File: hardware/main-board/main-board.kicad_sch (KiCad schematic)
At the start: 47 parts, among them J1 USB_C_Receptacle_USB2.0, J2 DNI, J3 Display Connector, U2 STM32L072KZT6, U4 USBLC6-2SC6, U5 TC1301A-APA

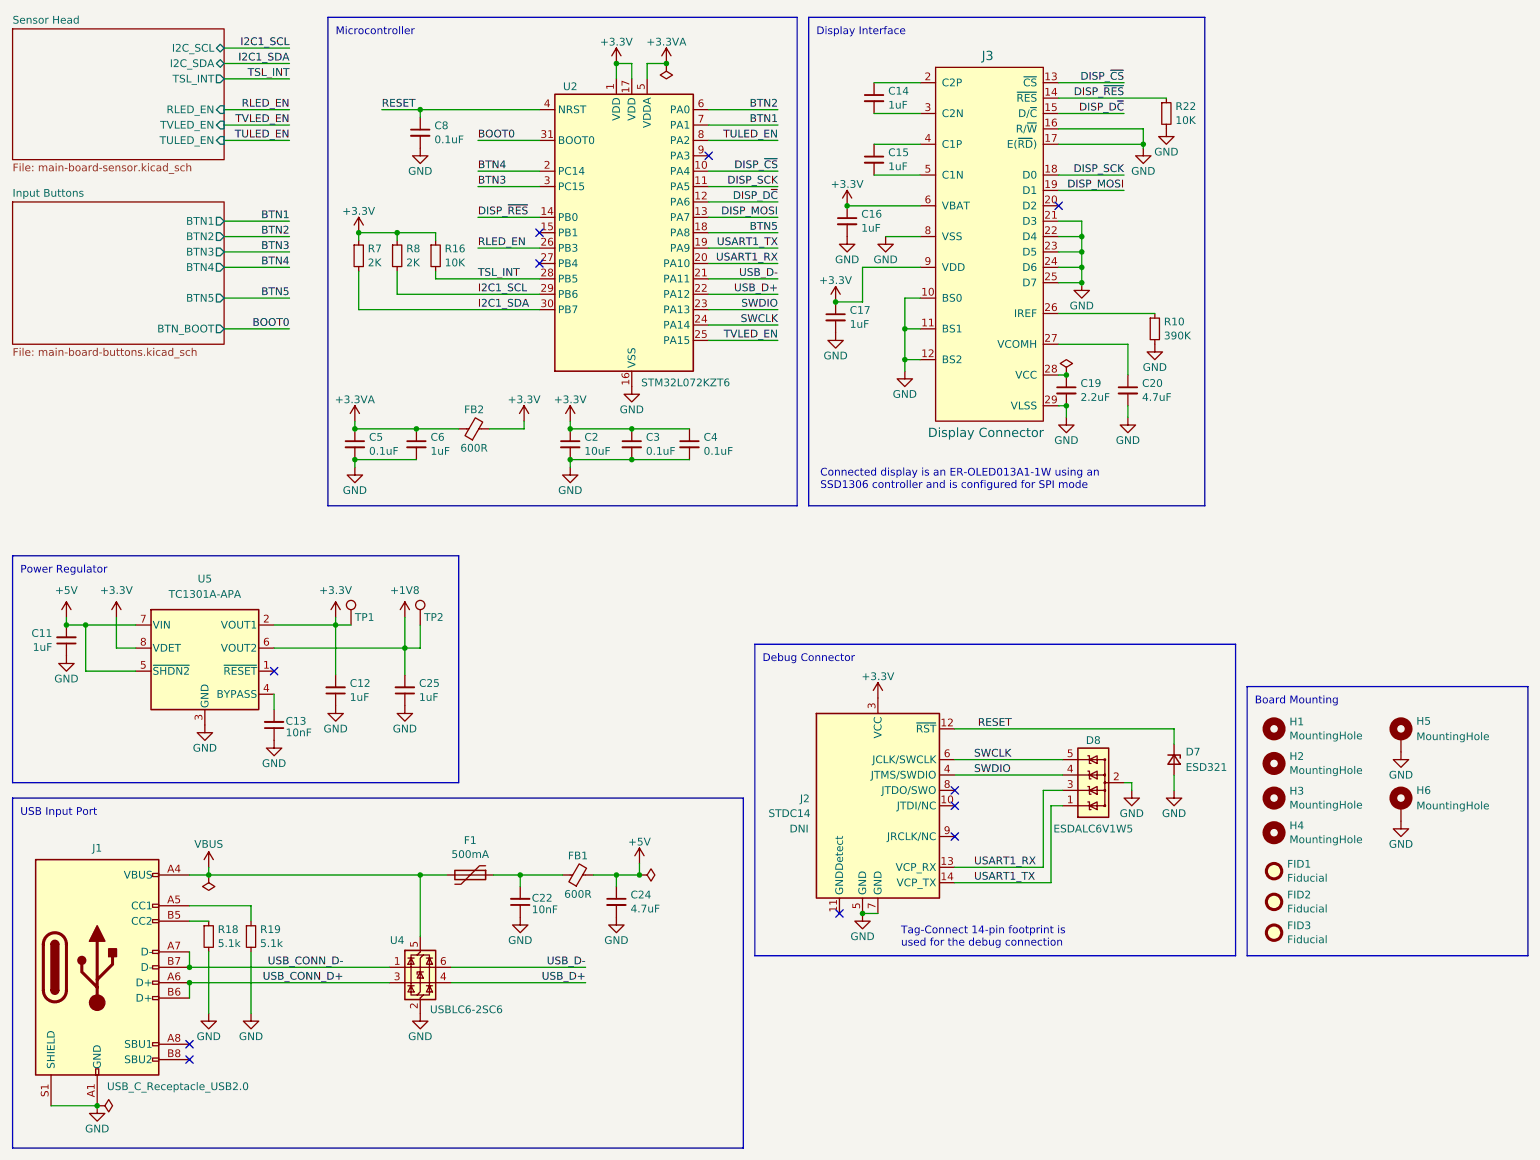
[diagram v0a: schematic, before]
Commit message: Final tweaks for Rev C manufacture
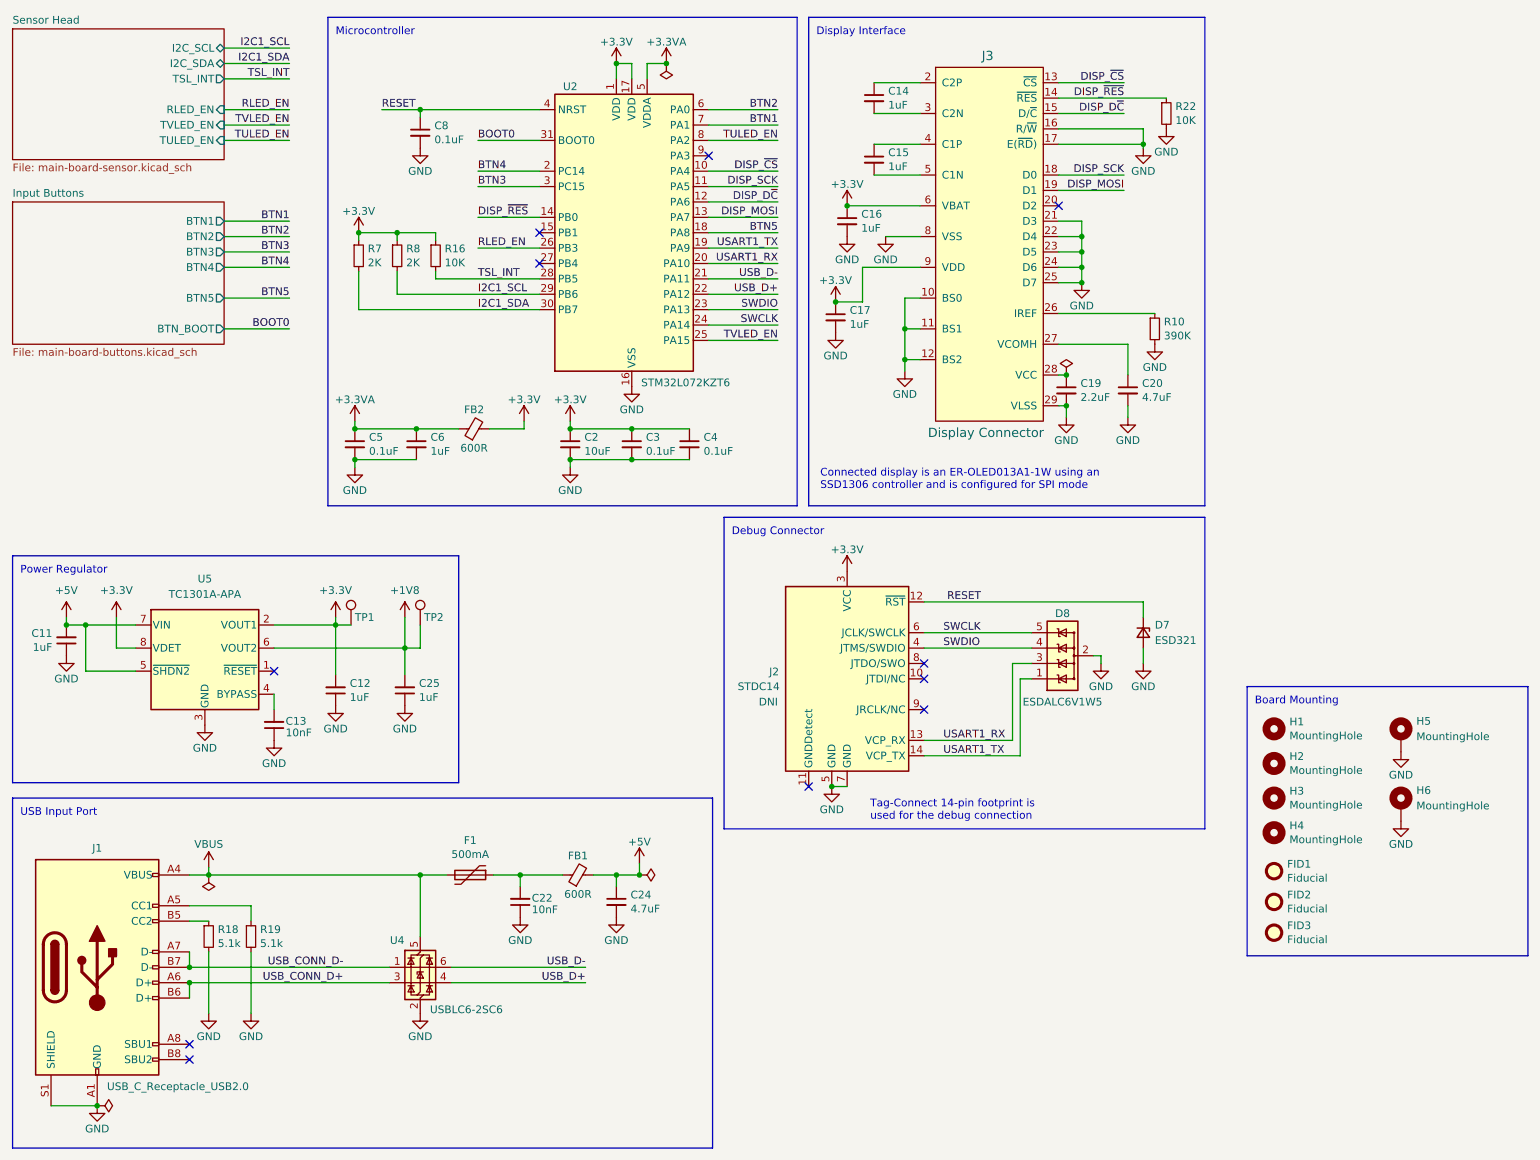
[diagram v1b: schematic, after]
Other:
- moved on the sheet: D7, D8, J2
